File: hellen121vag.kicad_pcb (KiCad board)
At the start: 4 copper layers, 164 x 118 mm, 102 parts, among them J21 Conn_01x05_Male, J22 USB_B_Mini, M1 Module-power_12and5V-0.3, M2 Module-knock-0.2, M3 Module-vr-discrete-0.5, M4 Module-vr-max9924-0.1, M5 Module-wbo-0.5, M6 Module:mega-mcu100/0.3, M7 Module-can-0.1, P1 368255-2, Q1 ISL9V3040D3ST, Q2 ISL9V3040D3ST, Q3 ISL9V3040D3ST, Q4 ISL9V3040D3ST, Q5 ISL9V3040D3ST, Q6 ISL9V3040D3ST, Q7 AO3400A, U10 BTS6143D, U11 VNLD5160TR-E, U3 VNLD5160TR-E, U4 VNLD5160TR-E, U5 VNLD5160TR-E, U6 VNLD5160TR-E, U7 VNLD5160TR-E, U8 MAX31855KASA, U9 VNLD5160TR-E

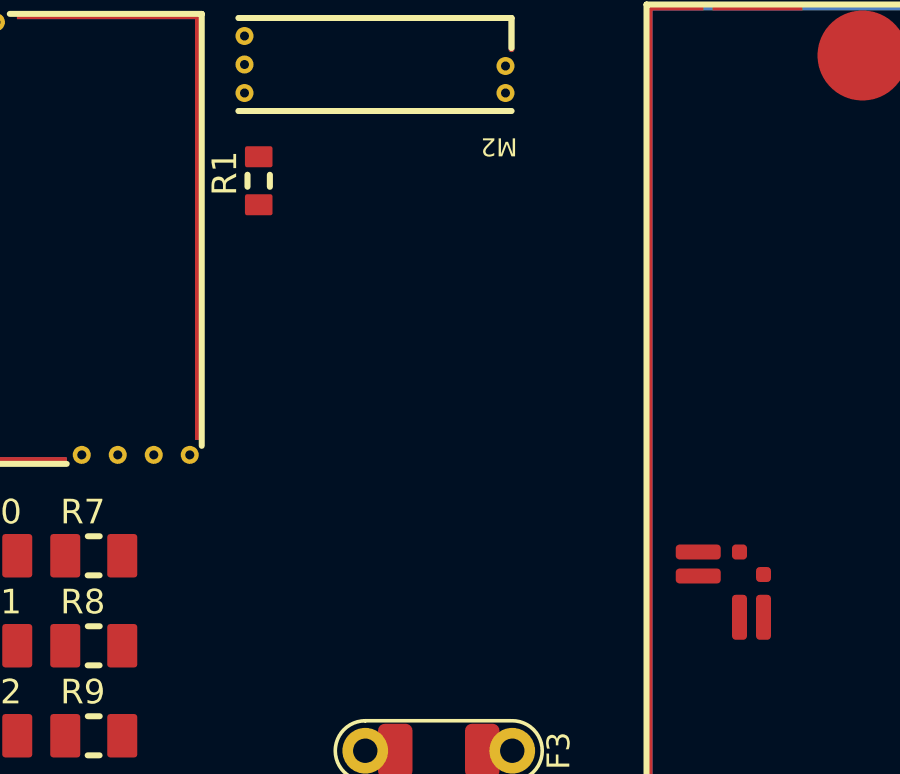
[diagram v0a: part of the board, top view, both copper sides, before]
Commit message: sw
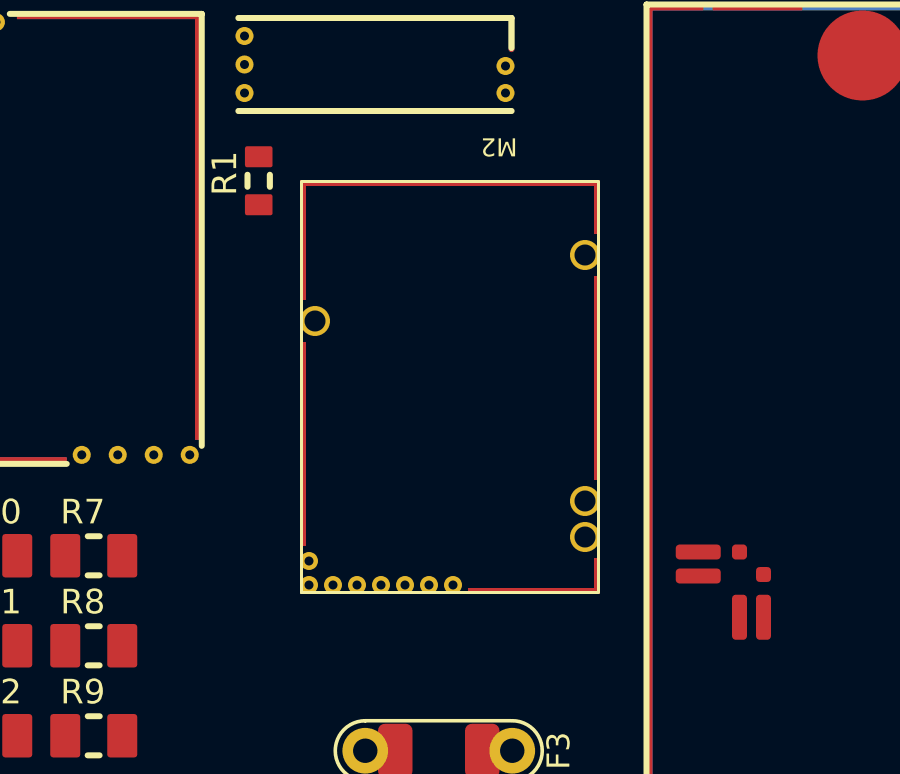
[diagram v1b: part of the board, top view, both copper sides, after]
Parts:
- added M8: Module-motor-driver-0.1, hellen-one-motor-driver-0.1:motor-driver, F.Cu at (166.9, 53.8)

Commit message: sw
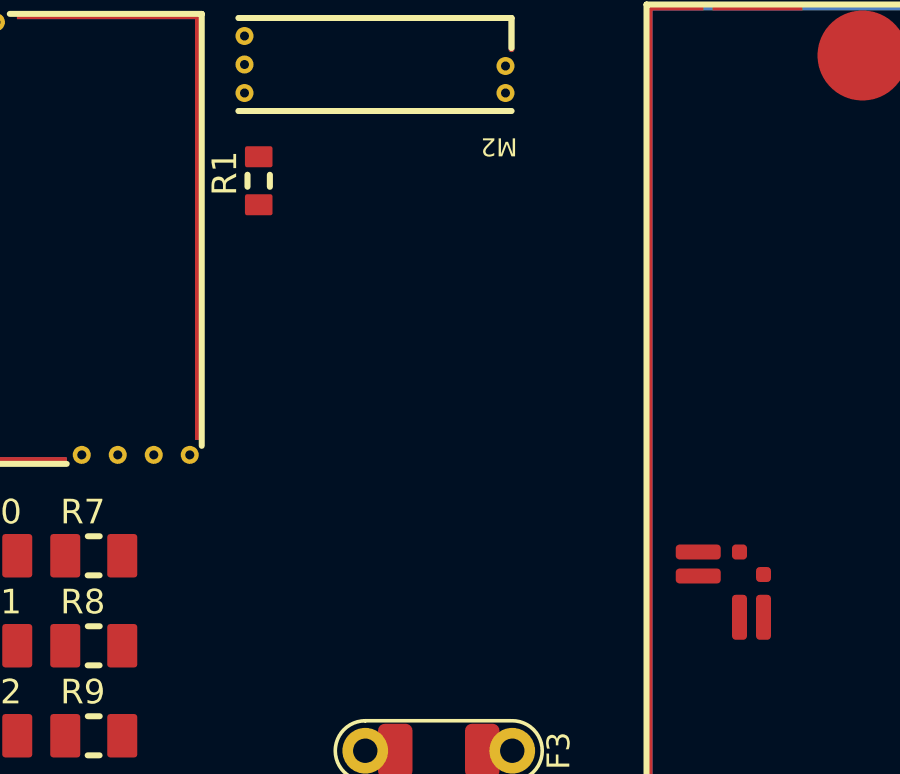
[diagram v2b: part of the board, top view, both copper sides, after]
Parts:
- removed M8: Module-motor-driver-0.1, hellen-one-motor-driver-0.1:motor-driver
